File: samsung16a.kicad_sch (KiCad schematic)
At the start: 0 parts

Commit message: Вибрав основний Чіп
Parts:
- added U?: STM32G431CBTx, Package_QFP:LQFP-48_7x7mm_P0.5mm, symbol MCU_ST_STM32G4:STM32G431CBTx
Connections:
- new net: U?.23 (VSS), U?.35 (VSS), U?.47 (VSS)
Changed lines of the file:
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@@
 	(generator_version "10.0")
 	(paper "A4")
+	(symbol
+		(lib_id "MCU_ST_STM32G4:STM32G431CBTx")
+		(at 152.4 102.87 0)
+		(unit 1)
+		(body_style 1)
+		(exclude_from_sim no)
+		(in_bom yes)
+		(on_board yes)
+		(in_pos_files yes)
+		(dnp no)
+		(fields_autoplaced yes)
+		(property "Reference" "U?"
+			(at 157.0833 143.51 0)
+			(show_name no)
+			(do_not_autoplace no)
+			(effects
+				(font
+					(size 1.27 1.27)
+				)
+				(justify left)
+			)
+		)
+		(property "Value" "STM32G431CBTx"
+			(at 157.0833 146.05 0)
+			(show_name no)
+			(do_not_autoplace no)
+			(effects
+				(font
+					(size 1.27 1.27)
+				)
+				(justify left)
+			)
+		)
+		(property "Footprint" "Package_QFP:LQFP-48_7x7mm_P0.5mm"
+			(at 137.16 140.97 0)
+			(hide yes)
+			(show_name no)
+			(do_not_autoplace no)
+			(effects
+				(font
+					(size 1.27 1.27)
+				)
+				(justify right)
+			)
+		)
+		(property "Datasheet" "https://www.st.com/resource/en/datasheet/stm32g431cb.pdf"
+			(at 152.4 102.87 0)
+			(hide yes)
+			(show_name no)
+			(do_not_autoplace no)
+			(effects
+				(font
+					(size 1.27 1.27)
+				)
+			)
+		)
+		(property "Description" "STMicroelectronics Arm Cortex-M4 MCU, 128KB flash, 32KB RAM, 170 MHz, 1.71-3.6V, 38 GPIO, LQFP48"
+			(at 152.4 102.87 0)
+			(hide yes)
+			(show_name no)
+			(do_not_autoplace no)
+			(effects
+				(font
+					(size 1.27 1.27)
+				)
+			)
+		)
+		(pin "4"
+		)
+		(pin "2"
+		)
+		(pin "3"
+		)
+		(pin "6"
+		)
+		(pin "7"
+		)
+		(pin "9"
+		)
+		(pin "5"
+		)
+		(pin "8"
+		)
+		(pin "1"
+		)
+		(pin "10"
+		)
+		(pin "11"
+		)
+		(pin "12"
+		)
+		(pin "13"
+		)
+		(pin "14"
+		)
+		(pin "15"
+		)
+		(pin "16"
+		)
+		(pin "20"
+		)
+		(pin "26"
+		)
+		(pin "27"
+		)
+		(pin "17"
+		)
+		(pin "22"
+		)
+		(pin "24"
+		)
+		(pin "25"
+		)
+		(pin "23"
+		)
+		(pin "18"
+		)
+		(pin "19"
+		)
+		(pin "21"
+		)
+		(pin "35"
+		)
+		(pin "28"
+		)
+		(pin "33"
+		)
+		(pin "29"
+		)
+		(pin "30"
+		)
+		(pin "31"
+		)
+		(pin "32"
+		)
+		(pin "34"
+		)
+		(pin "39"
+		)
+		(pin "36"
+		)
+		(pin "37"
+		)
+		(pin "38"
+		)
+		(pin "44"
+		)
+		(pin "43"
+		)
+		(pin "48"
+		)
+		(pin "41"
+		)
+		(pin "47"
+		)
+		(pin "42"
+		)
+		(pin "46"
+		)
+		(pin "45"
+		)
+		(pin "40"
+		)
+		(instances
+			(project "samsung16a"
+				(path "/1c8e70df-7651-4b9f-86c8-b2d78d9d3e27"
+					(reference "U?")
+					(unit 1)
+				)
+			)
+		)
+	)
 	(sheet_instances
 		(path "/"

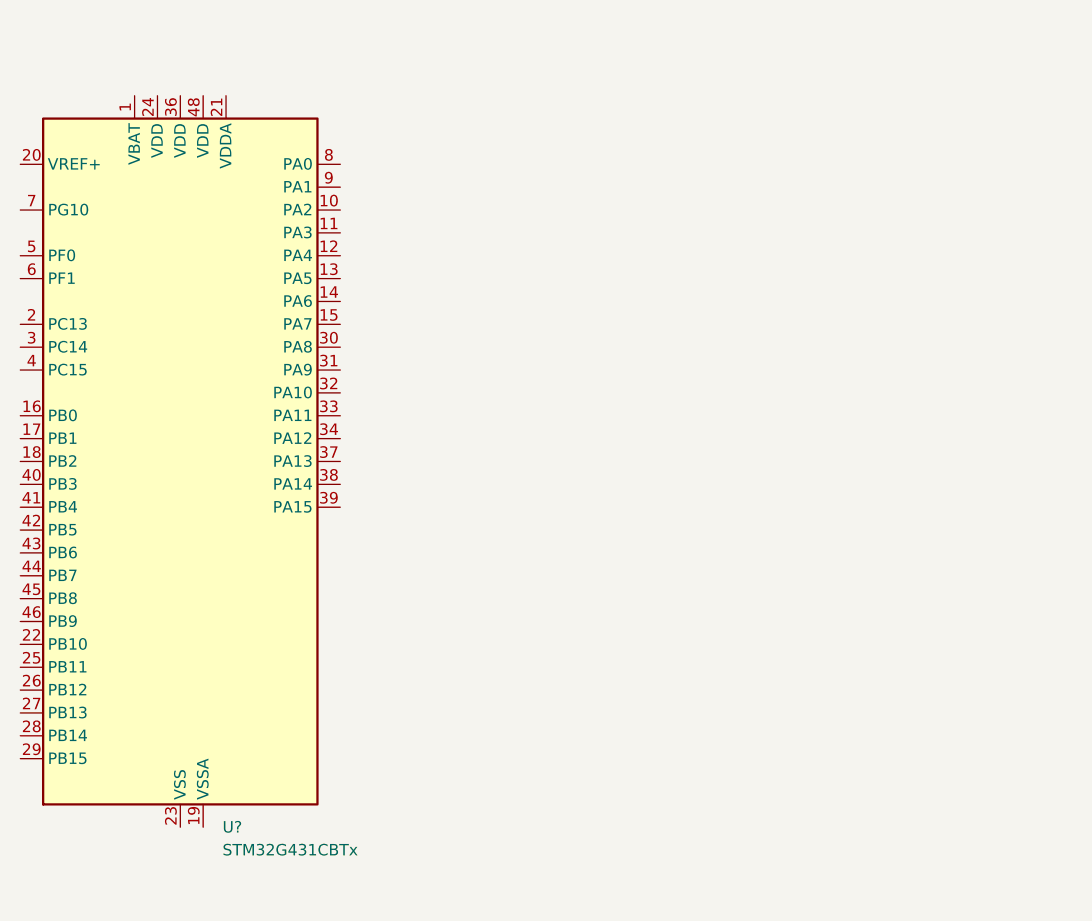
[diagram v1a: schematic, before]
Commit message: USB-C
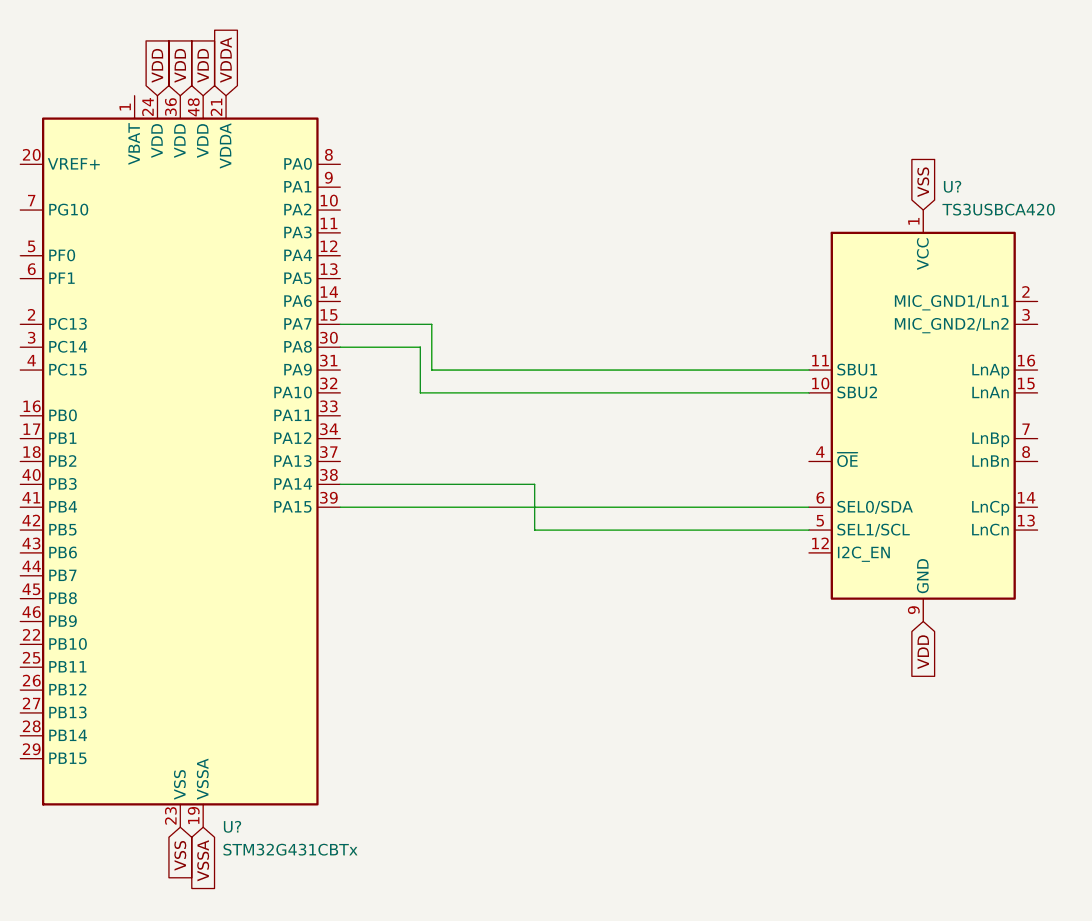
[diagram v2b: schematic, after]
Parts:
- added U?: TS3USBCA420, Package_DFN_QFN:UQFN-16_1.8x2.6mm_P0.4mm, symbol Interface_USB:TS3USBCA420
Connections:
- net at U?.15 (PA7): now also U?.11 (SBU1)
- net VSSA: now reaches U?.19 (VSSA)
- net VDDA: now reaches U?.21 (VDDA)
- net VSS: now reaches U?.23 (VSS), U?.35 (VSS), U?.47 (VSS)
- net VSS: now also U?.1 (VCC)
- net VDD: now reaches U?.24 (VDD)
- net VDD: now also U?.36 (VDD), U?.48 (VDD), U?.9 (GND)
- net at U?.30 (PA8): now also U?.10 (SBU2)
- net at U?.38 (PA14): now also U?.5 (SEL1/SCL)
- net at U?.39 (PA15): now also U?.6 (SEL0/SDA)
